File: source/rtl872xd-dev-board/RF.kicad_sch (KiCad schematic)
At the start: 18 parts, among them J1 Conn_Coaxial, U1 RTL8722DM

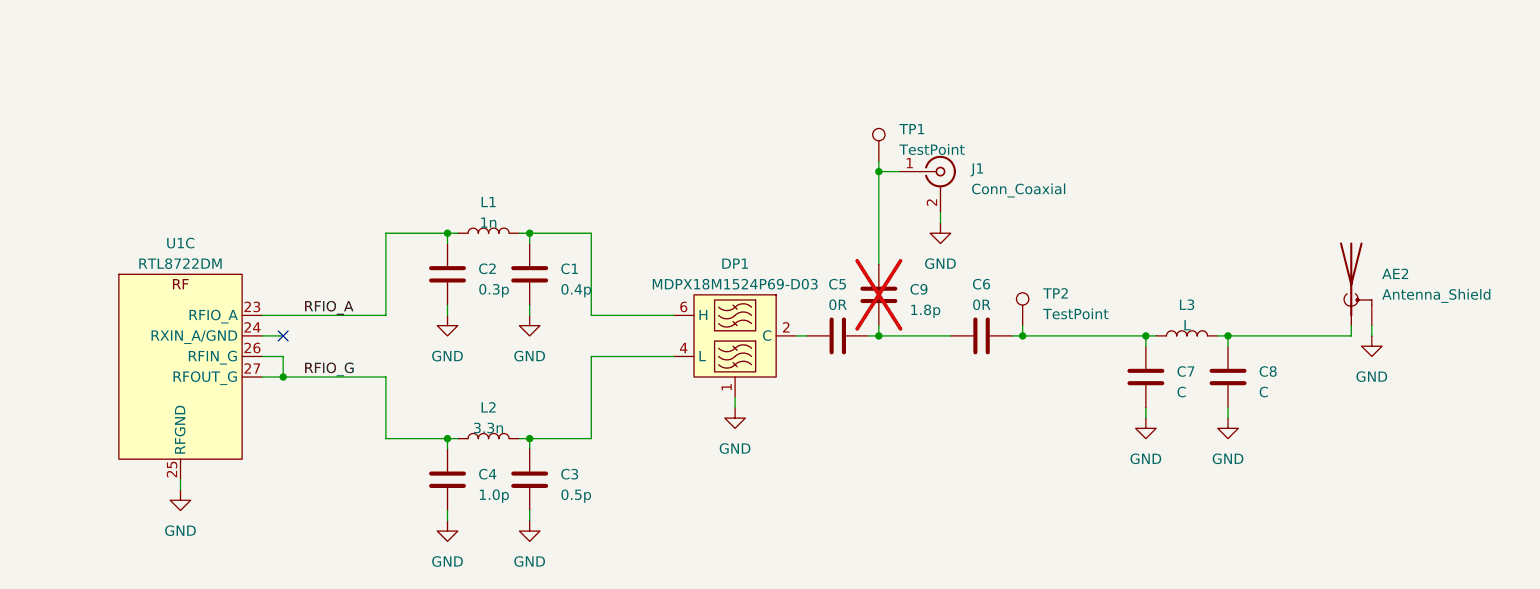
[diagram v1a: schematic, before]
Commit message: tidied up like Marie Kondo
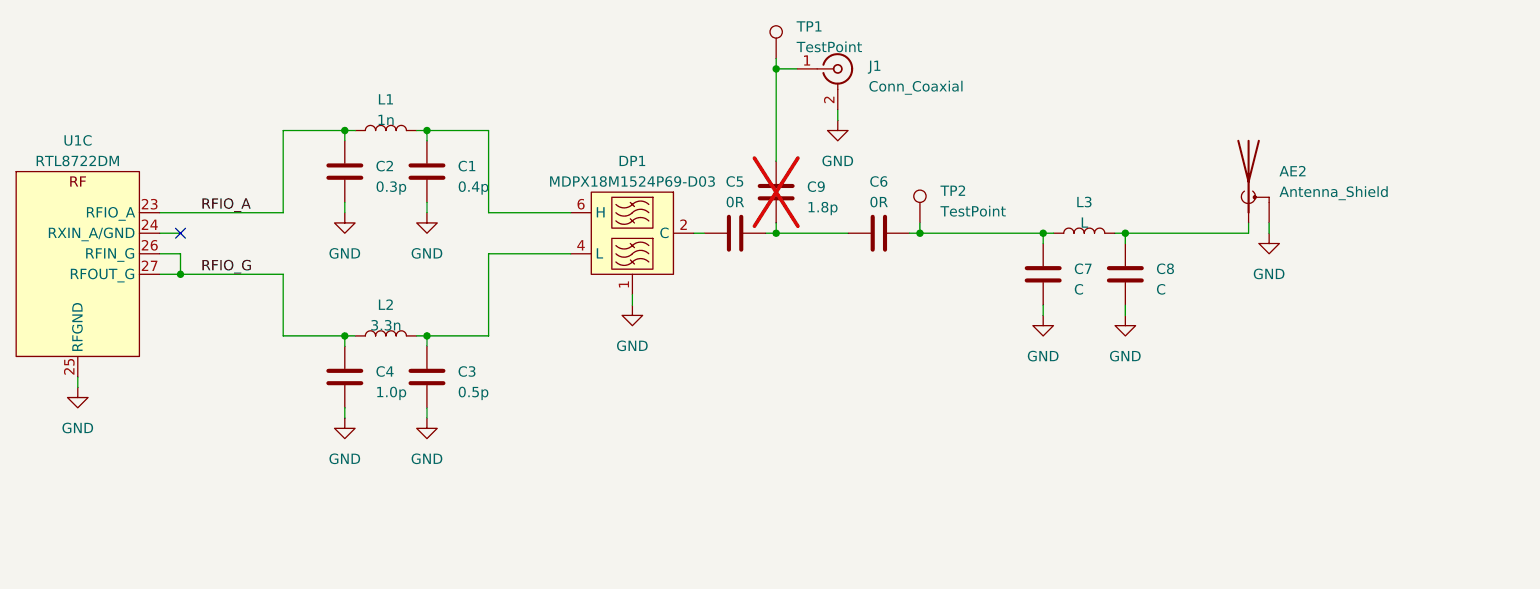
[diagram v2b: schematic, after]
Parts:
- C9: now left out of the parts list
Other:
- moved on the sheet: AE2, C1, C2, C3, C4, C5, C6, C7, C8, C9, DP1, J1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
